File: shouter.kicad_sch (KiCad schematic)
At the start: 27 parts, among them J1 Conn_01x02, J2 Conn_Coaxial, Q1 AO3422, Q2 AO3422, Q3 RGT16BM65DTL, SW1 SW_Push, T1 PE-68386NL, T2 PE-68386NL, U1 SFH601-2X007

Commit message: update components and footprints
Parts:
- C1, C2: PART_NUMBER_LCSC (none) -> C51205
- C3: PART_NUMBER_LCSC (none) -> C24497
- C4: PART_NUMBER_LCSC (none) -> C106147
- D1, D2, D3: footprint (none) -> Diode_SMD:Nexperia_CFP3_SOD-123W; PART_NUMBER_LCSC (none) -> C330237
- D4: PART_NUMBER_LCSC (none) -> C50432
- D5: footprint Diode_THT:D_DO-41_SOD81_P10.16mm_Horizontal -> Diode_SMD:Nexperia_CFP3_SOD-123W; PART_NUMBER_LCSC (none) -> C891584
- J2: footprint (none) -> Connector_Coaxial:SMA_Amphenol_132289_EdgeMount
- Q1, Q2: footprint Package_TO_SOT_SMD:TO-252-2 -> Package_TO_SOT_SMD:SOT-23; PART_NUMBER_LCSC (none) -> C37130
- Q3: PART_NUMBER_LCSC (none) -> C3193927
- R1: PART_NUMBER_LCSC (none) -> C1409
- R2: PART_NUMBER_LCSC (none) -> C71198
- R3, R4: PART_NUMBER_LCSC (none) -> C17954
- R5, R8: PART_NUMBER_LCSC (none) -> C17903
- R6, R7: PART_NUMBER_LCSC (none) -> C4410
- R9: PART_NUMBER_LCSC (none) -> C17944
- SW1: footprint (none) -> Button_Switch_SMD:SW_SPST_CK_RS282G05A3; PART_NUMBER_LCSC (none) -> C318938
- T1, T2: PART_NUMBER_LCSC (none) -> C581397
- U1: PART_NUMBER_LCSC (none) -> C17237090

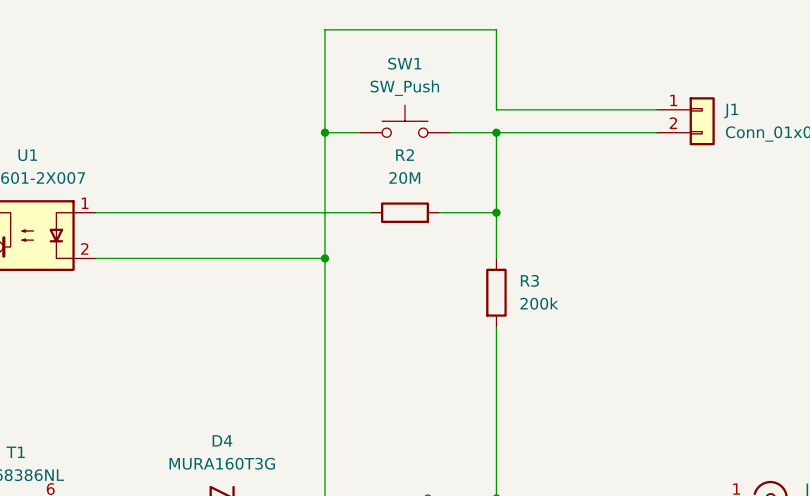
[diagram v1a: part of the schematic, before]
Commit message: 'pads_añadidos'
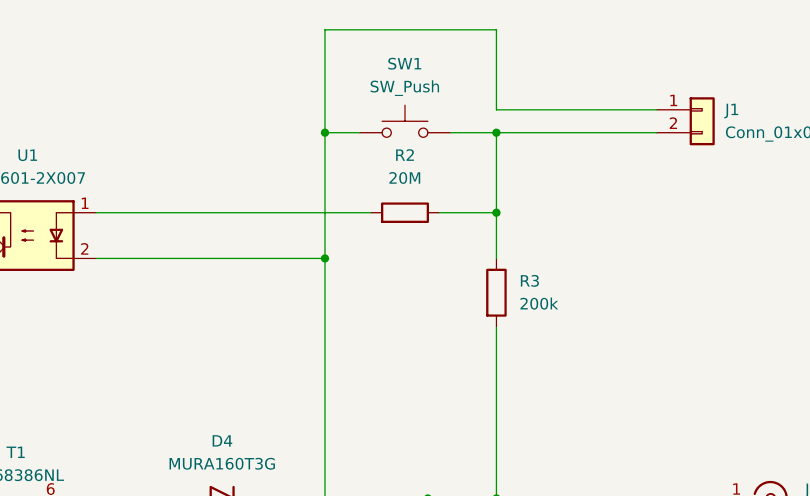
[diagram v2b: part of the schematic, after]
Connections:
- net at U1.1: now also R2.2; no longer R2.1
- net at J1.2 (Pin_2), R3.1, SW1.2: now also R2.1; no longer R2.2
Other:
- moved on the sheet: R2
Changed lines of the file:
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@@
 	(symbol
 		(lib_id "Device:R")
-		(at 173.99 50.8 90)
+		(at 173.99 50.8 270)
+		(mirror x)
 		(unit 1)
 		(exclude_from_sim no)
@@
 		(on_board yes)
 		(dnp no)
-		(fields_autoplaced yes)
 		(property "Reference" "R2"
 			(at 173.99 44.45 90)
